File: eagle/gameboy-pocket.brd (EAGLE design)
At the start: 69.5 x 117.2 mm, 32 parts, among them J1 AUDIO_JACK_3.5MM_PTH, U1 LM4875

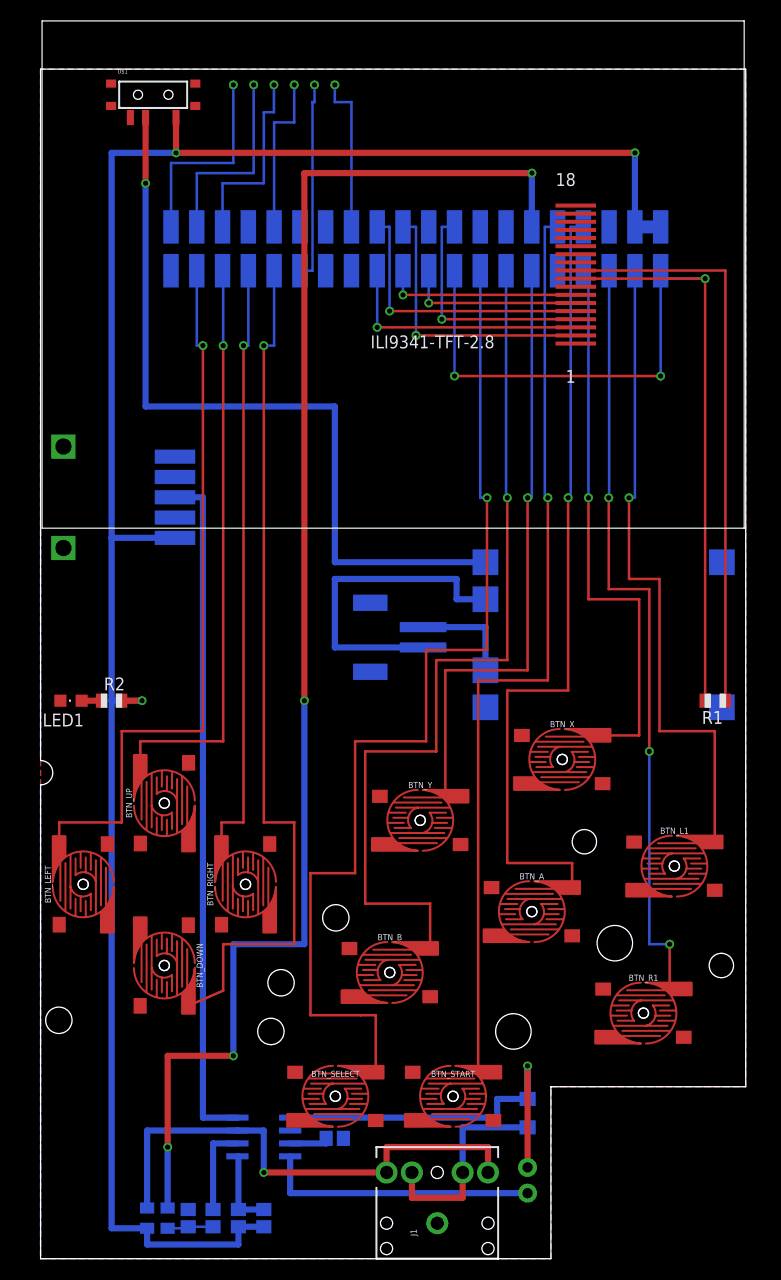
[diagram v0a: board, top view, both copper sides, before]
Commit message: Fri 22 Dec 2017 11:04:23 EST
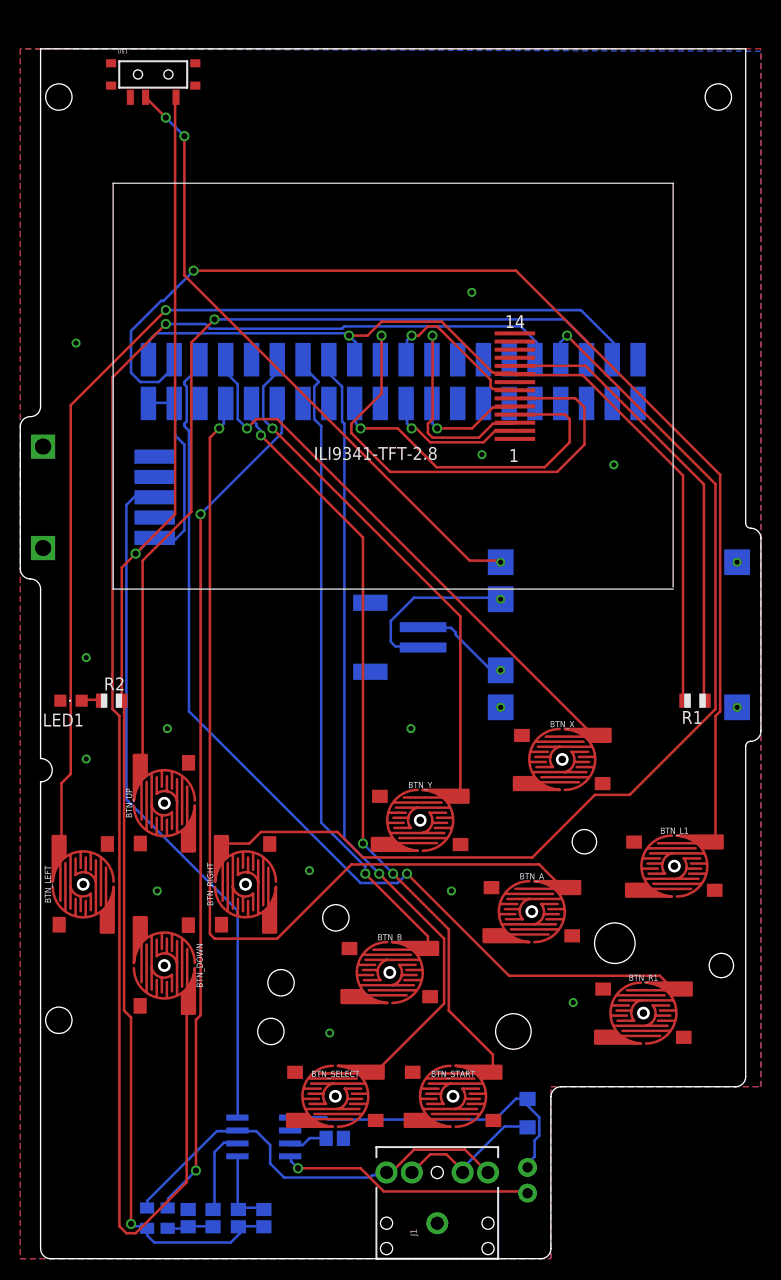
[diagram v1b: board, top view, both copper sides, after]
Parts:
- ILI9341-TFT-2.8: value GAMEBOYZEROHANDHELDDISPLAYS-2.8 -> GAMEBOYZEROHANDHELDDISPLAYS-2.2; device GameboyZeroHandheldDisplays:GAMEBOYZEROHANDHELDDISPLAYS-2.8 -> GameboyZeroHandheldDisplays:GAMEBOYZEROHANDHELDDISPLAYS-2.2
- moved PI1 78.2 mm to (2.25, 113.0), turned to 180 degrees
- moved ILI9341-TFT-2.8 11.0 mm to (34.8, 86.0)
- moved R1 2.00 mm to (64.5, 55.0)
- moved R10 2.00 mm to (9.25, 75.0)
- moved U$1 2.00 mm to (11.1, 116.7)
- moved POWER1 1.50 mm to (44.0, 53.0)
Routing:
- net DOWN: track 85.7 -> 157.2 mm
- net PWM: track 143.6 -> 84.2 mm, vias 4 -> 2
- net L1: track 65.3 -> 115.3 mm
- net SWITCH_OUT+: track 200.5 -> 150.6 mm, vias 3 -> 2
- net RIGHT: track 59.2 -> 101.8 mm
- net LEFT: track 71.3 -> 104.2 mm
- net SDI: track 17.7 -> 49.8 mm
- net UP: track 56.7 -> 86.3 mm
- net SELECT: track 103.5 -> 77.7 mm
- net B: track 87.3 -> 63.7 mm
- net GPIO21: track 20.1 -> 0.00 mm, vias 1 -> 0
- net GPIO5: track 19.8 -> 0.00 mm, vias 1 -> 0
- net GPIO20: track 19.6 -> 0.00 mm, vias 1 -> 0
- net GPIO16: track 19.1 -> 0.00 mm, vias 1 -> 0
- net R1: track 78.2 -> 96.6 mm, vias 3 -> 1
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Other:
- board size 69.5 x 117.2 mm -> 73 x 119.2 mm
